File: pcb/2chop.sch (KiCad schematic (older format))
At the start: 7 parts, among them U1 TL082

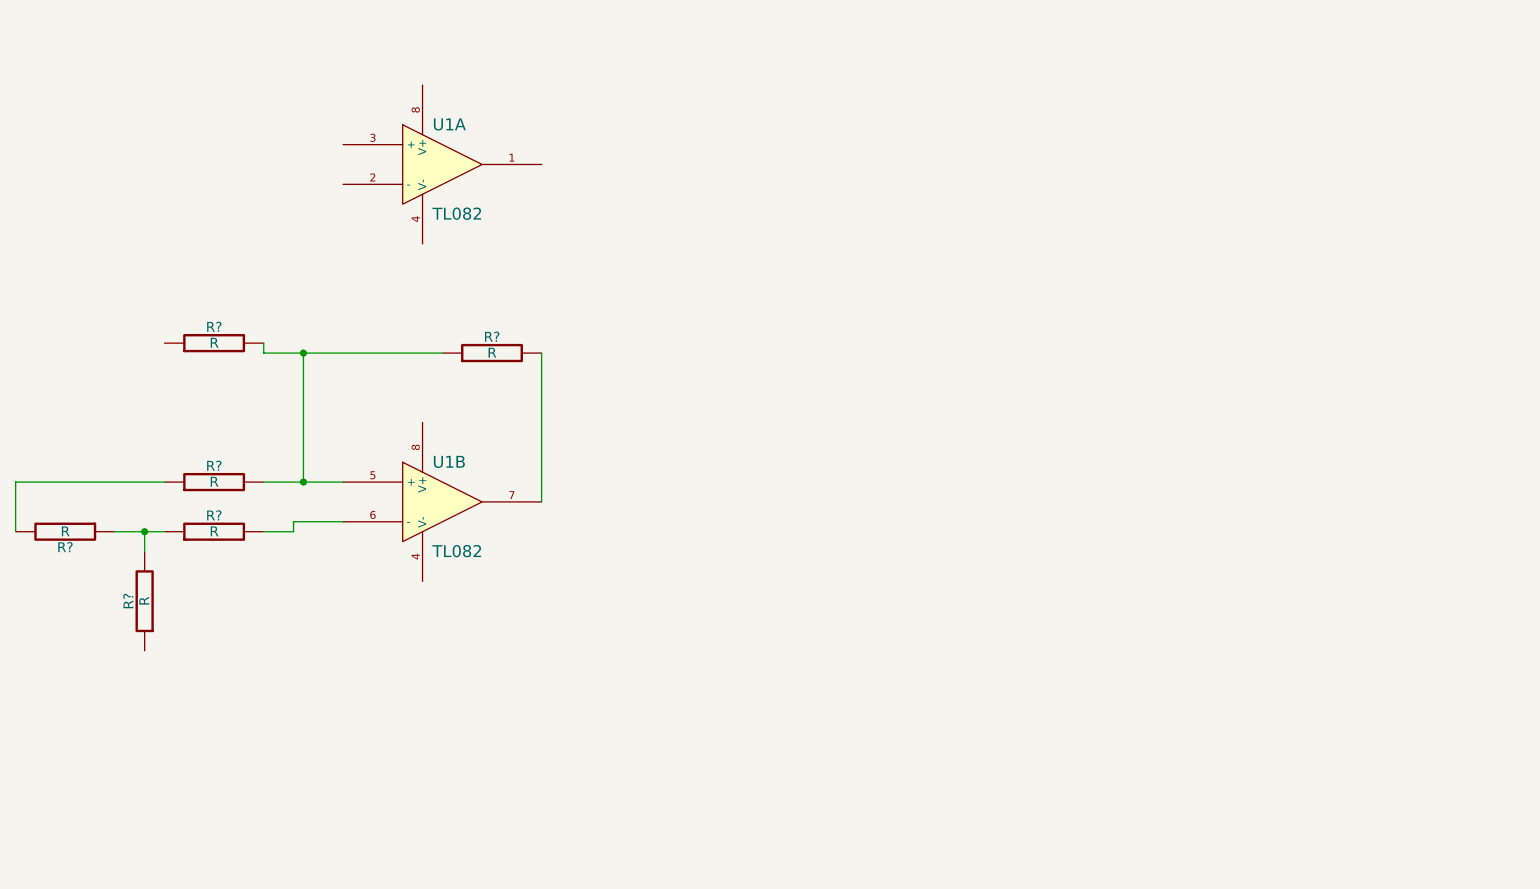
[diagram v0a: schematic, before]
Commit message: Schematic almost done
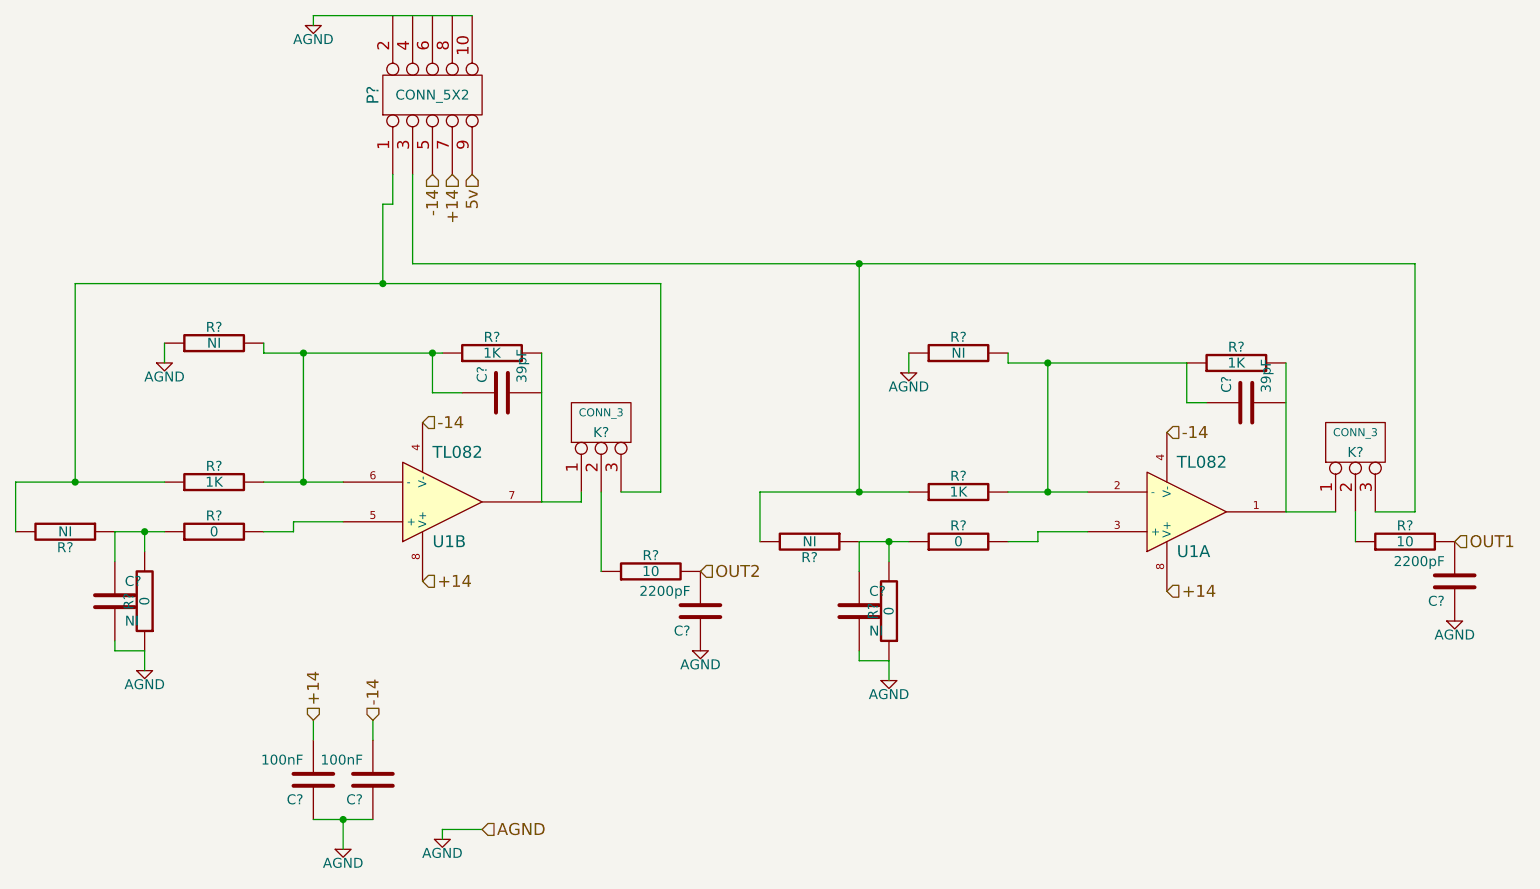
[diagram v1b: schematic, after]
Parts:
- added C? (x2): NI, symbol C
- added C? (x2): 39pF, symbol C
- added C? (x2): 100nF, symbol C
- added C? (x2): 2200pF, symbol C
- added K? (x2): CONN_3, symbol CONN_3
- added P?: CONN_5X2, symbol CONN_5X2
- added R? (x2): 1K, symbol R
- added R? (x2): NI, symbol R
- added R? (x2): 0, symbol R
- added R? (x2): 10, symbol R
- R? (x2): value R -> 1K
- R? (x2): value R -> NI
- R? (x2): value R -> 0
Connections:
- net at U1.1: now also K?.1 (P1), R?.2
- net at U1.2 (-): now also C?.1, R?.1, R?.2, R?.2
- net at U1.3 (+): now also R?.2
- net -14: now reaches U1.4 (V-)
- net -14: now also U1.4 (V-), C?.2, P?.5
- net +14: now reaches U1.8 (V+)
- net +14: now also U1.8 (V+), C?.2, P?.7
- net at R?.1, R?.2, R?.2: now also U1.6 (-), C?.1; no longer U1.5 (+)
- net at R?.2: now also U1.5 (+); no longer U1.6 (-)
- net at R?.2, U1.7: now also K?.1 (P1)
- net AGND: now reaches R?.1
- net AGND: now also R?.1, C?.1, C?.1, C?.1, C?.1, C?.2, C?.2, P?.10, R?.1, R?.1
- net at R?.1, R?.2: now also K?.3 (P3), P?.1
- net at R?.1, R?.1, R?.2: now also C?.1
- new net: K?.3 (P3), P?.3, R?.1, R?.2
- new net: C?.1, R?.1, R?.1, R?.2
- new net: K?.2 (PM), R?.1 (x2)
- new net 5v: P?.9
- new net OUT1: C?.2, R?.2
- new net OUT2: C?.2, R?.2
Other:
- moved on the sheet: U1A
